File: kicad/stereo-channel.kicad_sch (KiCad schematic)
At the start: 13 parts, among them U2 TL072

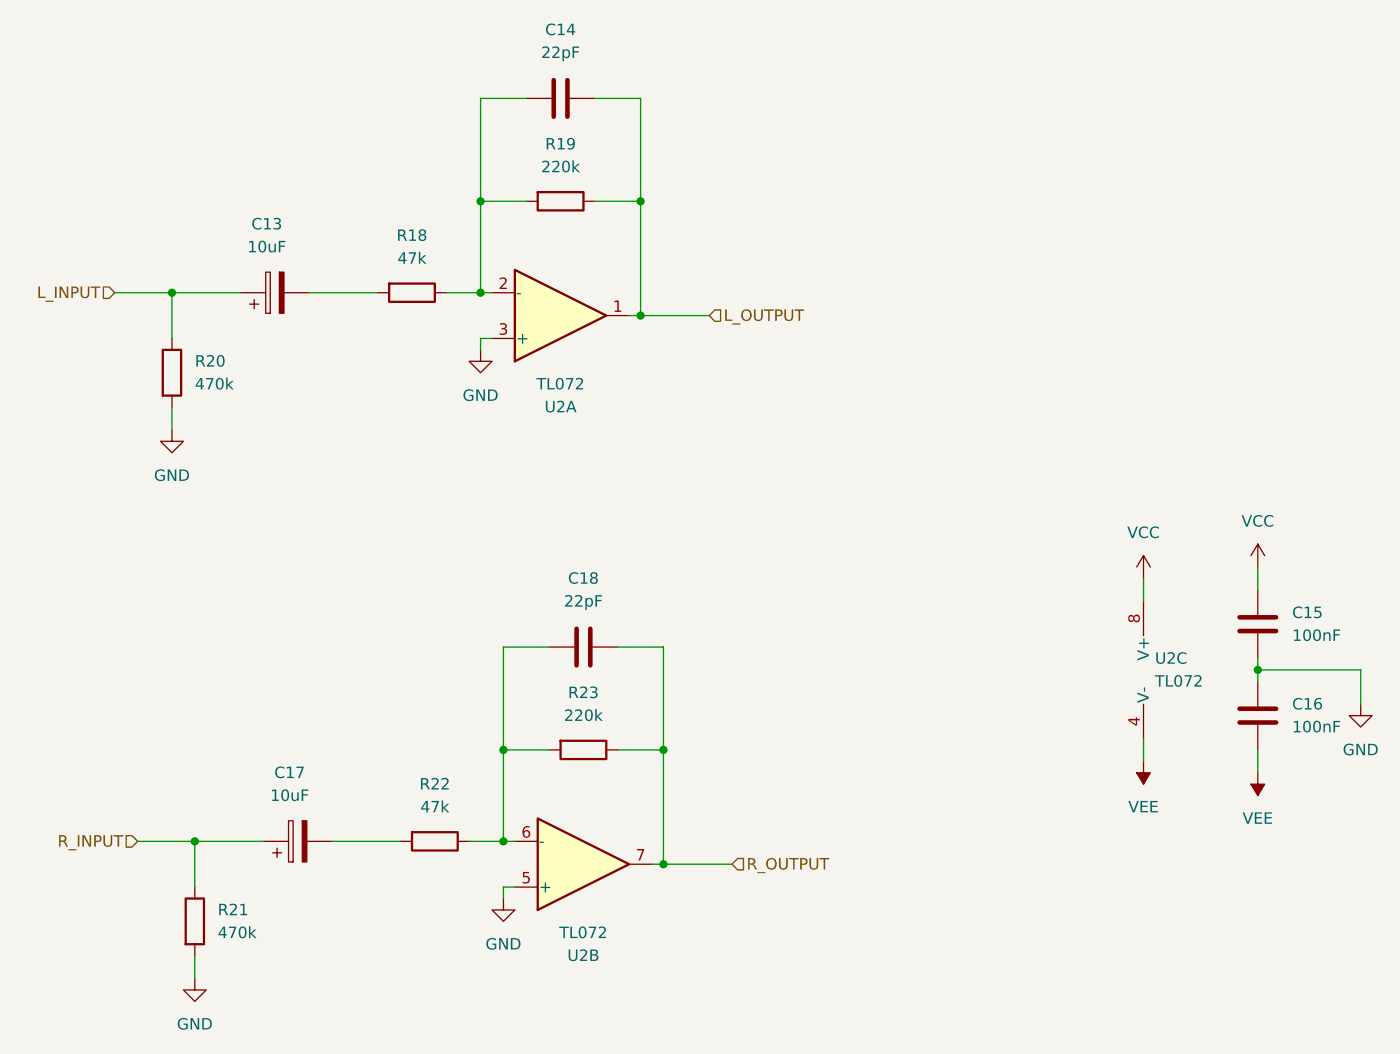
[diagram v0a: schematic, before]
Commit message: Updating everything and adding gerbers
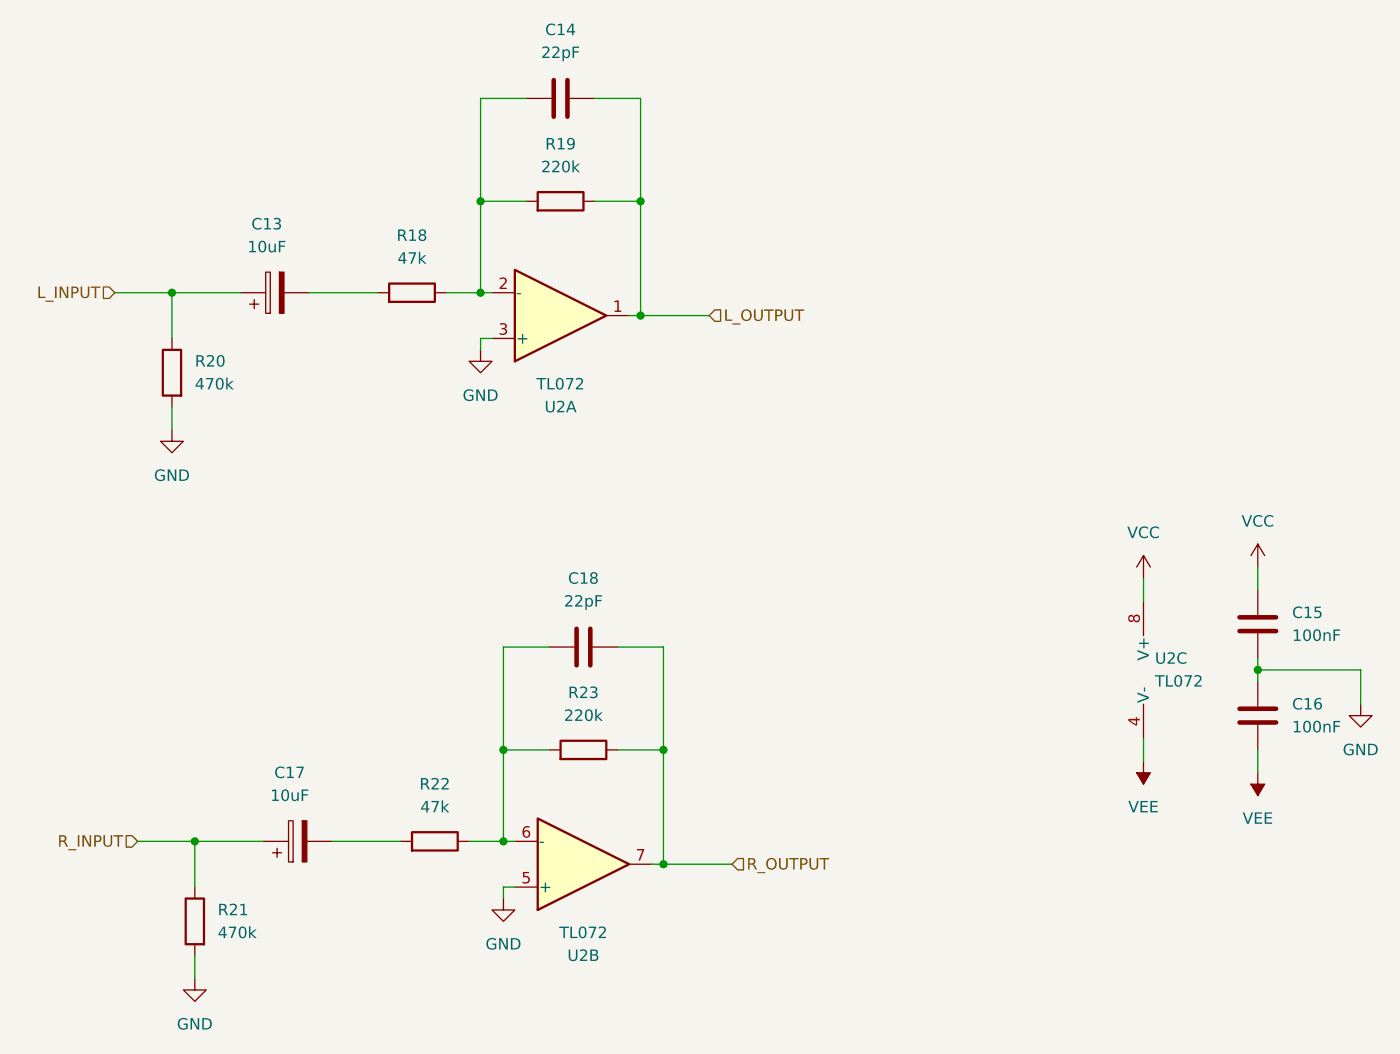
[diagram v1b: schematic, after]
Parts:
- C13, C17: footprint Capacitor_THT:CP_Radial_D5.0mm_P2.00mm -> Rumblesan_Standard_Parts:CP_Radial_D5.0mm_P2.00mm; symbol Standard_Parts:C_Polarized -> Rumblesan_Standard_Parts:C_Polarized
- C14, C15, C16, C18: symbol Standard_Parts:C -> Rumblesan_Standard_Parts:C
- R18, R19, R20, R21, R22, R23: symbol Standard_Parts:R -> Rumblesan_Standard_Parts:R
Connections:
- net GND: now also R20.1, R21.1; no longer R20.2, R21.2
- net L_INPUT: now also R20.2; no longer R20.1
- net L_OUTPUT: now also R19.2; no longer R19.1
- net R_INPUT: now also R21.2; no longer R21.1
- net R_OUTPUT: now also R23.2; no longer R23.1
- net at C18.1, U2.6 (-): now also R22.2, R23.1; no longer R22.1, R23.2
- net at C13.2: now also R18.1; no longer R18.2
- net at C14.1, U2.2 (-): now also R18.2, R19.1; no longer R18.1, R19.2
- net at C17.2: now also R22.1; no longer R22.2
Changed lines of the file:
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@@
 	)
 	(symbol
-		(lib_id "Standard_Parts:R")
+		(lib_id "Rumblesan_Standard_Parts:R")
 		(at 120.65 127 90)
 		(unit 1)
@@
 	)
 	(symbol
-		(lib_id "Standard_Parts:R")
+		(lib_id "Rumblesan_Standard_Parts:R")
 		(at 74.93 85.09 180)
 		(unit 1)
@@
 	)
 	(symbol
-		(lib_id "Standard_Parts:C_Polarized")
+		(lib_id "Rumblesan_Standard_Parts:C_Polarized")
 		(at 86.36 76.2 90)
 		(unit 1)
@@
 			)
 		)
-		(property "Footprint" "Capacitor_THT:CP_Radial_D5.0mm_P2.00mm"
+		(property "Footprint" "Rumblesan_Standard_Parts:CP_Radial_D5.0mm_P2.00mm"
 			(at 86.36 69.85 90)
 			(effects
@@
 	)
 	(symbol
-		(lib_id "Standard_Parts:C")
+		(lib_id "Rumblesan_Standard_Parts:C")
 		(at 118.11 54.61 90)
 		(unit 1)
@@
 	)
 	(symbol
-		(lib_id "Standard_Parts:R")
+		(lib_id "Rumblesan_Standard_Parts:R")
 		(at 101.6 76.2 90)
 		(unit 1)
@@
 	)
 	(symbol
-		(lib_id "Standard_Parts:R")
+		(lib_id "Rumblesan_Standard_Parts:R")
 		(at 77.47 146.05 180)
 		(unit 1)
@@
 	)
 	(symbol
-		(lib_id "Standard_Parts:C")
+		(lib_id "Rumblesan_Standard_Parts:C")
 		(at 195.58 123.19 180)
 		(unit 1)
@@
 	)
 	(symbol
-		(lib_id "Standard_Parts:R")
+		(lib_id "Rumblesan_Standard_Parts:R")
 		(at 104.14 137.16 90)
 		(unit 1)
@@
 	)
 	(symbol
-		(lib_id "Standard_Parts:C")
+		(lib_id "Rumblesan_Standard_Parts:C")
 		(at 195.58 113.03 180)
 		(unit 1)
@@
 	)
 	(symbol
-		(lib_id "Standard_Parts:C_Polarized")
+		(lib_id "Rumblesan_Standard_Parts:C_Polarized")
 		(at 88.9 137.16 90)
 		(unit 1)
@@
 			)
 		)
-		(property "Footprint" "Capacitor_THT:CP_Radial_D5.0mm_P2.00mm"
+		(property "Footprint" "Rumblesan_Standard_Parts:CP_Radial_D5.0mm_P2.00mm"
 			(at 88.9 130.81 90)
 			(effects
@@
 	)
 	(symbol
-		(lib_id "Standard_Parts:C")
+		(lib_id "Rumblesan_Standard_Parts:C")
 		(at 120.65 115.57 90)
 		(unit 1)
@@
 	)
 	(symbol
-		(lib_id "Standard_Parts:R")
+		(lib_id "Rumblesan_Standard_Parts:R")
 		(at 118.11 66.04 90)
 		(unit 1)
